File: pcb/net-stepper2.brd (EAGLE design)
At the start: 41.9 x 90.2 mm, 41 parts, among them IC2 CP2104, J1 MICRO-USB, J2 POWER_JACKPTH_LOCK, J3 ENCODER, J4 ENDSTOP2, J5 ENDSTOP1, J6 STEPER, Q1 600mA/40V, Q2 600mA/40V, U1 L6470, U2 ESP-WROOM-03, U3 RGB-LED, U4 TRACO12433

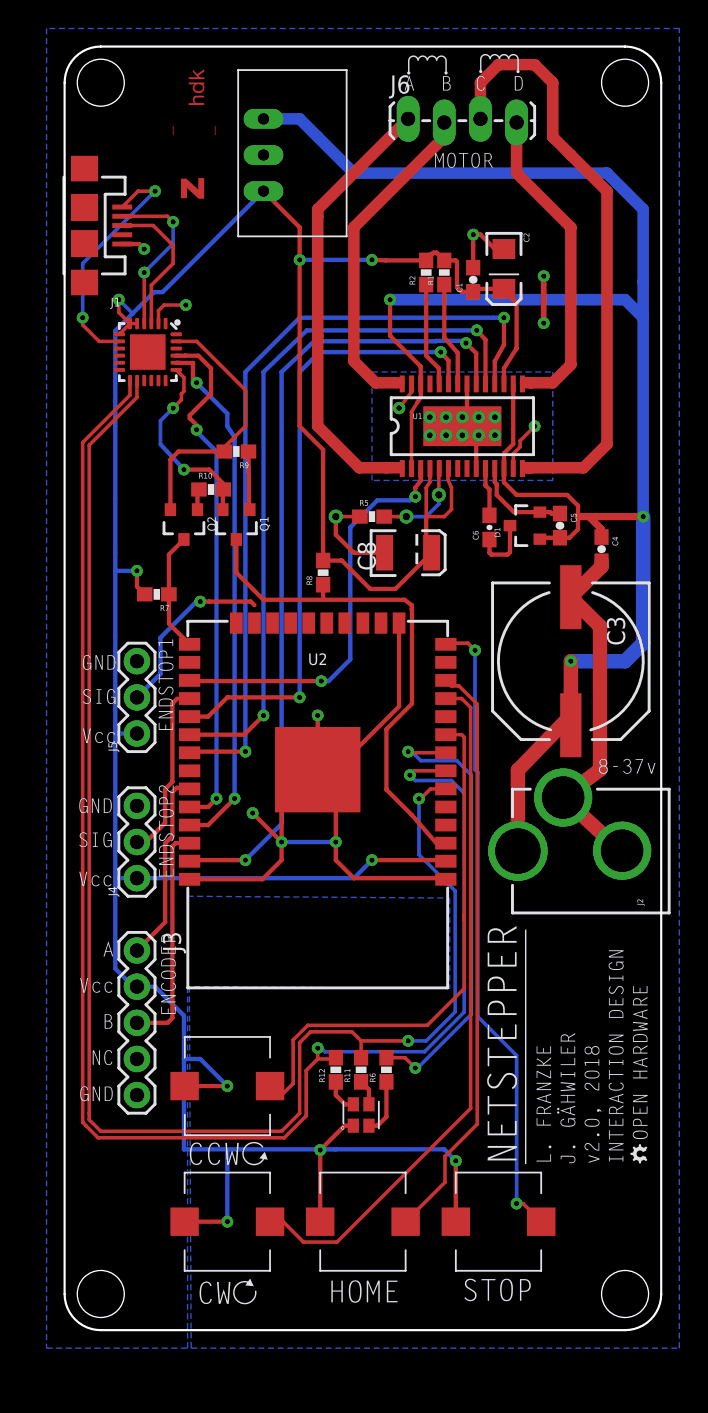
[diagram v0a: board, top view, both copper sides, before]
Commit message: moved board
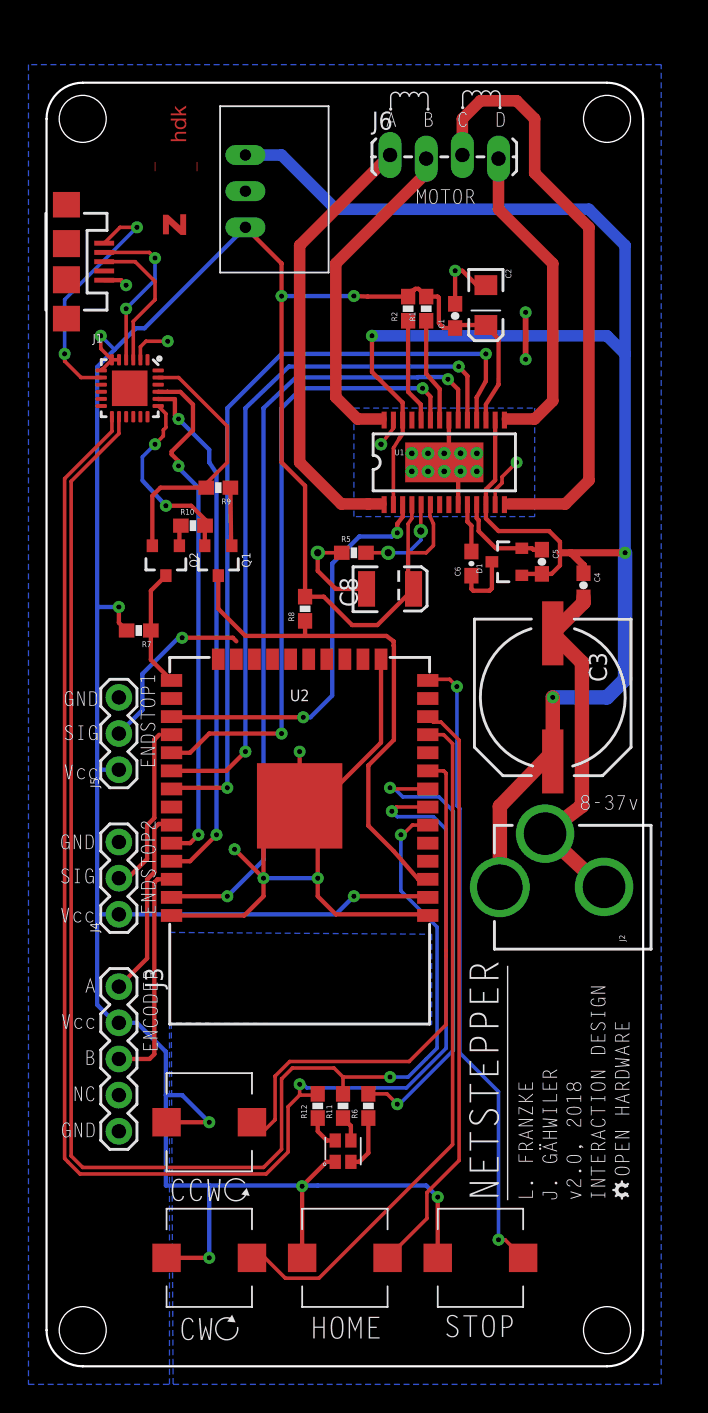
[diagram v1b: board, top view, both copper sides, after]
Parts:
- moved U$11 2.84 mm to (39.4, 87.6)
- moved A1 2.84 mm to (7.62, 78.7)
- moved IC2 2.84 mm to (5.84, 68.7)
- moved J1 2.84 mm to (1.40, 77.6)
- moved J5 2.84 mm to (5.08, 41.9)
- moved U$12 2.84 mm to (2.54, 87.6)
- moved U1 2.84 mm to (27.9, 63.5)
- moved U4 2.84 mm to (14.0, 82.5)
- moved C4 2.84 mm to (37.7, 54.9)
- moved S4 2.84 mm to (21.0, 7.62)
- moved U$10 2.84 mm to (39.4, 2.54)
- moved A2 2.84 mm to (2.54, 2.54)
- moved D1 2.84 mm to (32.4, 56.5)
- moved J2 2.84 mm to (45.7, 33.7)
- moved U$9 2.84 mm to (2.54, 2.54)
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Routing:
- net OUT1B: track 42.9 -> 42.3 mm
